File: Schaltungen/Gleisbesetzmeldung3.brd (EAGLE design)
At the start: 73 parts, among them IC1 CNY-17-2, IC10 S462, IC11 CNY-17-2, IC12 S462, IC13 CNY-17-2, IC14 S462, IC15 CNY-17-2, IC16 S462, IC2 S462, IC3 CNY-17-2, IC4 S462, IC5 CNY-17-2, IC6 S462, IC7 CNY-17-2, IC8 S462, IC9 CNY-17-2

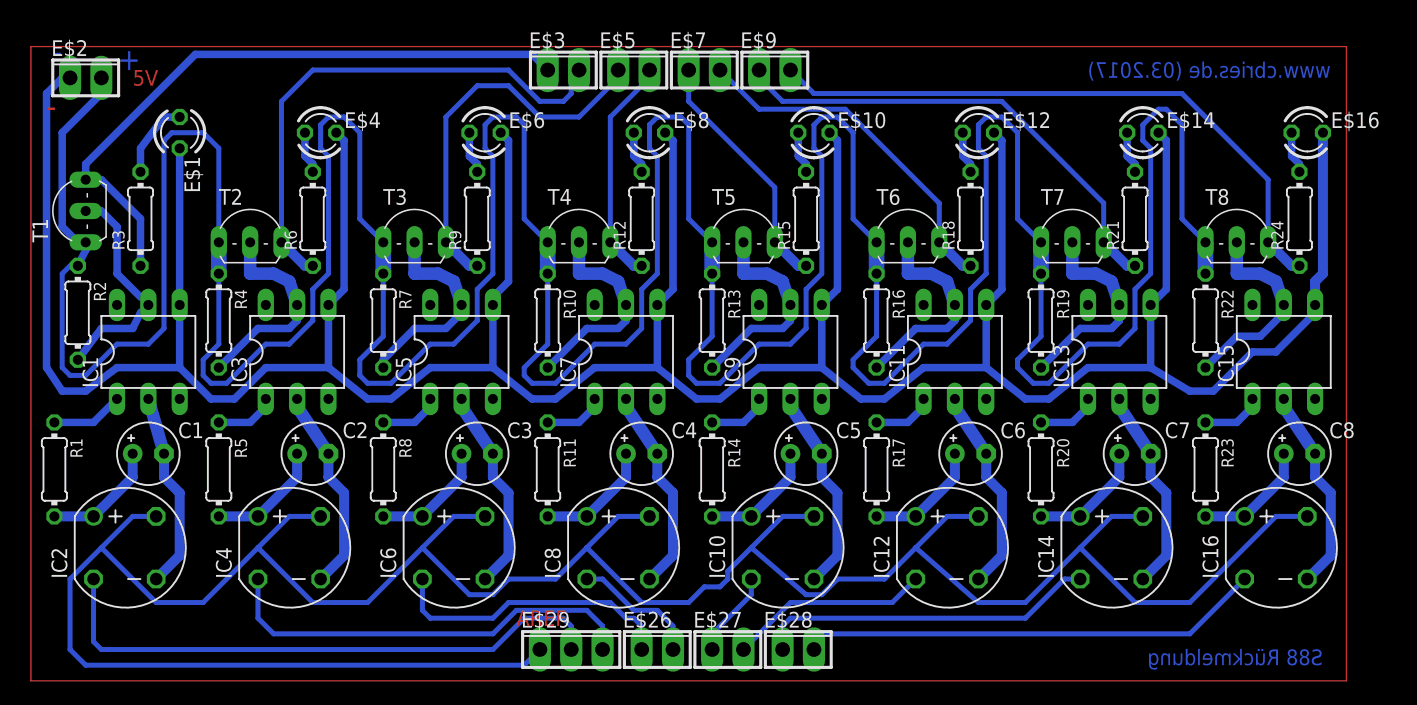
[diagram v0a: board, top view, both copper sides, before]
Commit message: gerber files
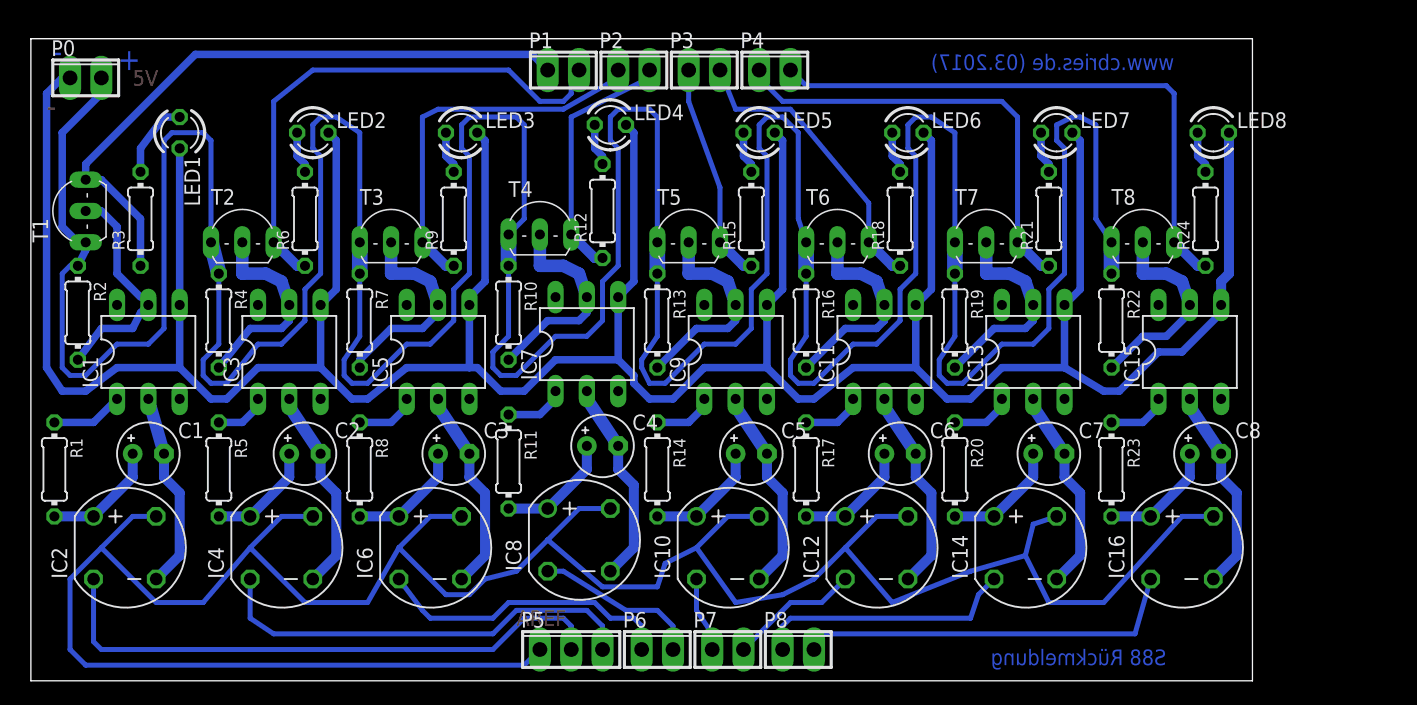
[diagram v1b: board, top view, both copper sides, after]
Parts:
- removed E$10, E$12, E$14, E$16, E$4, E$6, E$8: (no value), led:LED3MM
- added LED2, LED3, LED4, LED5, LED6, LED7, LED8: (no value), led:LED3MM
- moved C8 7.62 mm to (95.2, 18.4)
- moved IC16 7.62 mm to (93.3, 10.8)
- moved R22 7.62 mm to (87.6, 29.2)
- moved R23 7.62 mm to (87.6, 17.1)
- moved R24 7.62 mm to (95.2, 37.5)
- moved T8 7.62 mm to (90.2, 35.6)
- moved IC15 7.62 mm to (94.0, 26.7)
- moved C7 6.98 mm to (82.5, 18.4)
- moved IC13 6.98 mm to (81.3, 26.7)
- moved IC14 6.98 mm to (80.6, 10.8)
- moved R19 6.98 mm to (74.9, 29.2)
- moved R20 6.98 mm to (74.9, 17.1)
- moved R21 6.98 mm to (82.5, 37.5)
- moved T7 6.98 mm to (77.5, 35.6)
- moved C6 5.72 mm to (70.5, 18.4)
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- renumbered E$1 to LED1, E$2 to P0, E$26 to P6, E$27 to P7, E$28 to P8, E$29 to P5, E$3 to P1, E$5 to P2, E$7 to P3, E$9 to P4
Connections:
- net S$5: now also LED2.A, LED2.K, LED3.A, LED3.K, LED4.A, LED4.K, LED5.A, LED5.K, LED6.A, LED6.K, LED7.A, LED7.K, LED8.A, LED8.K; no longer E$10.A, E$10.K, E$12.A, E$12.K, E$14.A, E$14.K, E$16.A, E$16.K, E$4.A, E$4.K, E$6.A, E$6.K, E$8.A, E$8.K
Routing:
- net S$1: track 316.2 -> 0.00 mm
- net S$162: track 552.3 -> 528.9 mm
- net S$5: track 605.5 -> 588.0 mm
- net S$3: track 409.2 -> 403.2 mm
- net S$6: track 9.57 -> 8.94 mm
- net S$11: track 4.97 -> 4.34 mm
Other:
- board outline added: 99.1 x 52.1 mm
